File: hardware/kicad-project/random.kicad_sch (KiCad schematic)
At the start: 33 parts, among them J7 Conn_01x50, Q3 DMG2301L-7, SW10 TS-1135-C, SW4 K2-1109SP-C4SA, SW5 K2-1109SP-C4SA, SW6 K2-1109SP-C4SA, SW7 K2-1109SP-C4SA, SW8 TS-1135-C, SW9 TS-1135-C

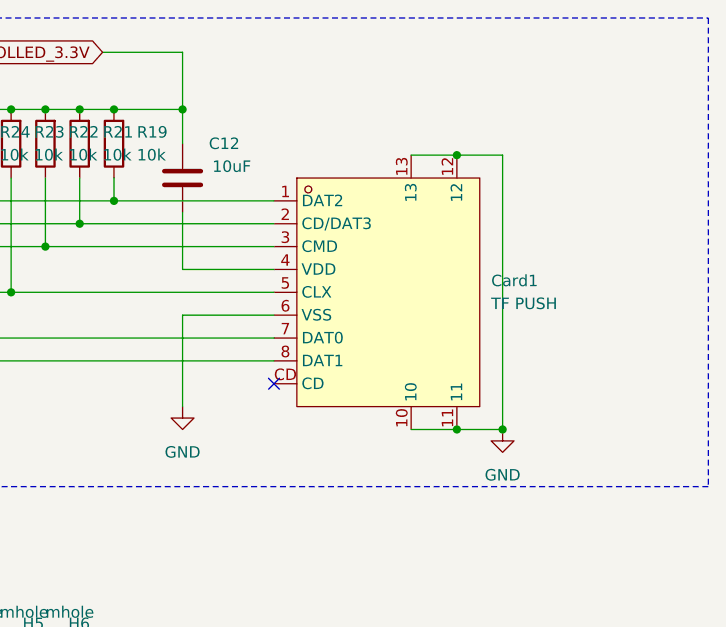
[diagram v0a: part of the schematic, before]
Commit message: wip
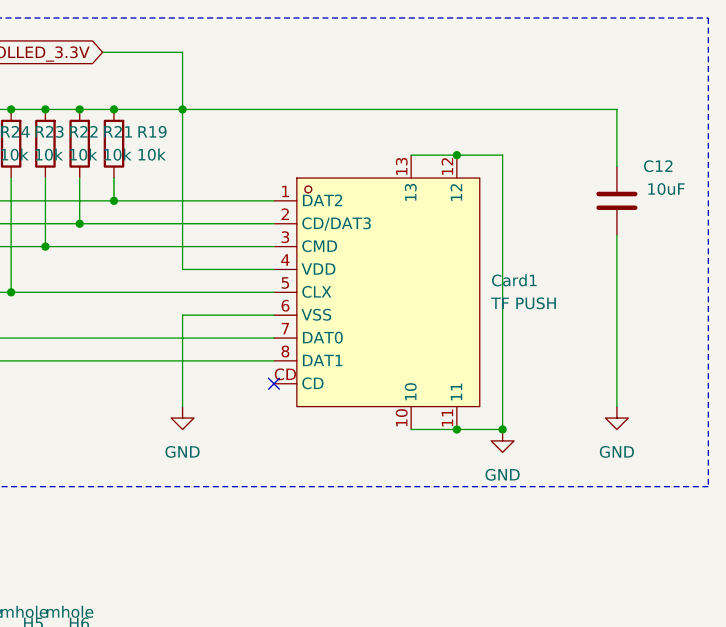
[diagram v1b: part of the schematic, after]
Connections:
- net +VSW: now also Card1.4 (VDD)
- net GND: now also C12.1
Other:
- moved on the sheet: C12
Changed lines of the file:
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@@
-    (stroke (width 0) (type default))
-  )
-  (wire (pts (xy 223.52 39.37) (xy 223.52 45.72))
     (stroke (width 0) (type default))
   )
@@
     (stroke (width 0) (type default))
   )
+  (wire (pts (xy 271.78 27.94) (xy 223.52 27.94))
+    (stroke (width 0) (type default))
+  )
   (wire (pts (xy 212.09 91.44) (xy 215.9 91.44))
     (stroke (width 0) (type default))
@@
     (stroke (width 0) (type default))
   )
-  (wire (pts (xy 223.52 27.94) (xy 223.52 31.75))
+  (wire (pts (xy 271.78 27.94) (xy 271.78 34.29))
     (stroke (width 0) (type default))
   )
@@
     (stroke (width 0) (type default))
   )
+  (wire (pts (xy 271.78 41.91) (xy 271.78 60.96))
+    (stroke (width 0) (type default))
+  )
   (wire (pts (xy 57.15 166.37) (xy 57.15 170.18))
     (stroke (width 0) (type default))
@@
   )
   (wire (pts (xy 135.89 29.21) (xy 144.78 29.21))
+    (stroke (width 0) (type default))
+  )
+  (wire (pts (xy 223.52 27.94) (xy 223.52 45.72))
     (stroke (width 0) (type default))
   )
@@
     )
   )
-  (symbol (lib_id "Device:C") (at 223.52 35.56 0) (mirror x) (unit 1)
-    (in_bom yes) (on_board yes) (dnp no)
-    (property "Reference" "C12" (at 229.87 31.75 0)
-      (effects (font (size 1.27 1.27)) (justify right))
-    )
-    (property "Value" "10uF" (at 231.14 34.29 0)
-      (effects (font (size 1.27 1.27)) (justify right))
-    )
-    (property "Footprint" "Capacitor_SMD:C_0805_2012Metric" (at 224.4852 31.75 0)
-      (effects (font (size 1.27 1.27)) hide)
-    )
-    (property "Datasheet" "~" (at 223.52 35.56 0)
+  (symbol (lib_id "Device:C") (at 271.78 38.1 0) (mirror x) (unit 1)
+    (in_bom yes) (on_board yes) (dnp no)
+    (property "Reference" "C12" (at 278.13 34.29 0)
+      (effects (font (size 1.27 1.27)) (justify right))
+    )
+    (property "Value" "10uF" (at 279.4 36.83 0)
+      (effects (font (size 1.27 1.27)) (justify right))
+    )
+    (property "Footprint" "Capacitor_SMD:C_0805_2012Metric" (at 272.7452 34.29 0)
+      (effects (font (size 1.27 1.27)) hide)
+    )
+    (property "Datasheet" "~" (at 271.78 38.1 0)
       (effects (font (size 1.27 1.27)) hide)
     )
@@
         )
       )
+    )
+  )
+  (symbol (lib_id "power:GND") (at 271.78 60.96 0) (mirror y) (unit 1)
+    (in_bom yes) (on_board yes) (dnp no)
+    (property "Reference" "#PWR062" (at 271.78 67.31 0)
+      (effects (font (size 1.27 1.27)) hide)
+    )
+    (property "Value" "GND" (at 271.78 66.04 0)
+      (effects (font (size 1.27 1.27)))
+    )
+    (property "Footprint" "" (at 271.78 60.96 0)
+      (effects (font (size 1.27 1.27)) hide)
+    )
+    (property "Datasheet" "" (at 271.78 60.96 0)
+      (effects (font (size 1.27 1.27)) hide)
+    )
+    (pin "1")
+    (instances
+      (project "Untitled"
+        (path "/0de5ae84-7f75-4a5a-83a1-35d27fd1d8d2"
+          (reference "#PWR062") (unit 1)
+        )
+        (path "/0de5ae84-7f75-4a5a-83a1-35d27fd1d8d2/7a3aed0a-25fa-4aa7-ba6a-02a8683cfb94"
+          (reference "#PWR014") (unit 1)
+        )
+      )
